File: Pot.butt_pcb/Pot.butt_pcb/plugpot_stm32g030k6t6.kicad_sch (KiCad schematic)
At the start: 12 parts, among them J1 Conn_01x04_Male, J2 Conn_01x05_Male, SW1 SW_Push, U1 STM32G030K6T6

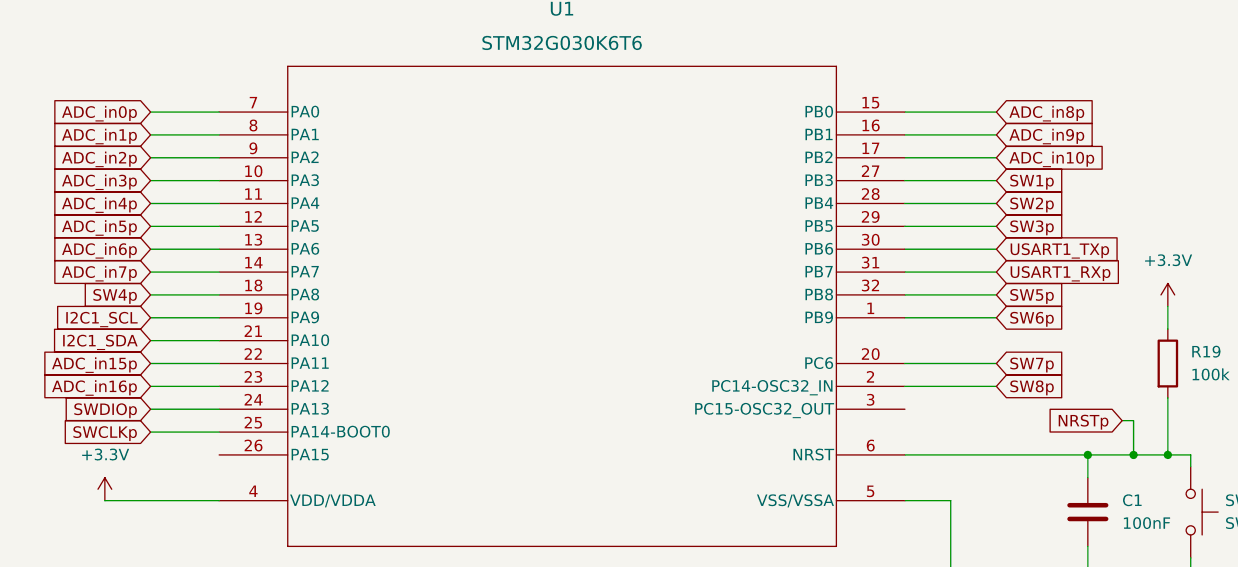
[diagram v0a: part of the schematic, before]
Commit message: Pot.but_pcb in progress
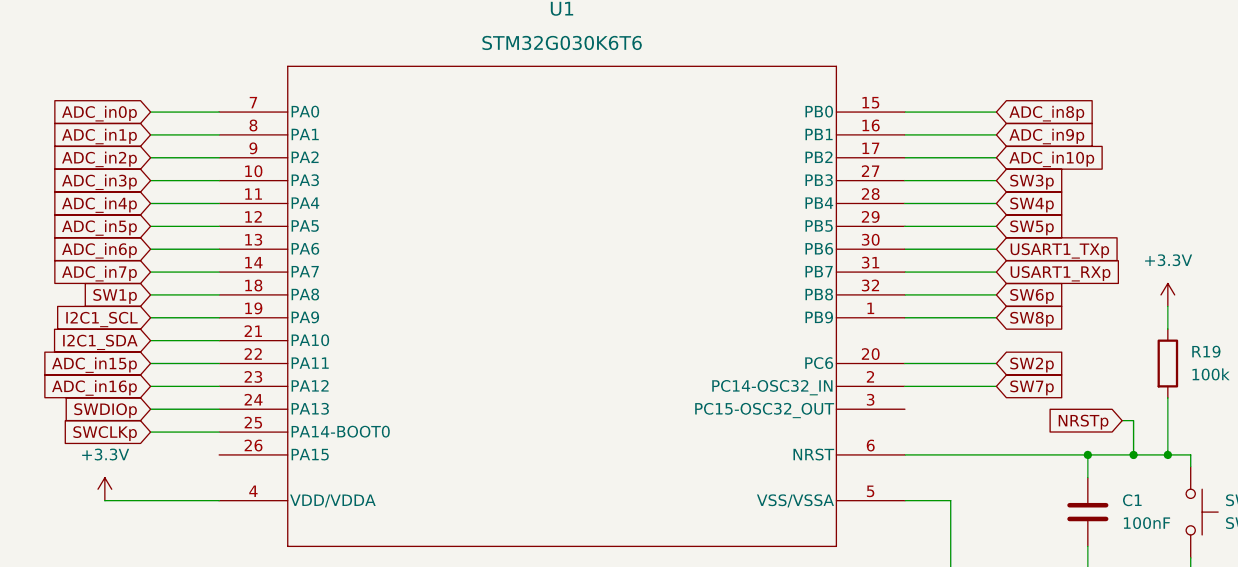
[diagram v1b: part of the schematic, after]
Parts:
- J1: footprint Connector_PinSocket_2.54mm:PinSocket_1x04_P2.54mm_Horizontal -> Connector_PinSocket_2.54mm:PinSocket_1x04_P2.54mm_Vertical
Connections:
- net SW1p: now also U1.18 (PA8); no longer U1.27 (PB3)
- net SW2p: now also U1.20 (PC6); no longer U1.28 (PB4)
- net SW3p: now also U1.27 (PB3); no longer U1.29 (PB5)
- net SW4p: now also U1.28 (PB4); no longer U1.18 (PA8)
- net SW5p: now also U1.29 (PB5); no longer U1.32 (PB8)
- net SW6p: now also U1.32 (PB8); no longer U1.1 (PB9)
- net SW7p: now also U1.2 (PC14-OSC32_IN); no longer U1.20 (PC6)
- net SW8p: now also U1.1 (PB9); no longer U1.2 (PC14-OSC32_IN)
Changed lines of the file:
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@@
     )
   )
-  (global_label "SW2p" (shape input) (at 137.16 60.96 0) (fields_autoplaced)
+  (global_label "SW4p" (shape input) (at 137.16 60.96 0) (fields_autoplaced)
     (effects (font (size 1.27 1.27)) (justify left))
     (property "Intersheet References" "${INTERSHEET_REFS}" (id 0) (at 144.5926 60.8806 0)
@@
     )
   )
-  (global_label "SW3p" (shape input) (at 137.16 63.5 0) (fields_autoplaced)
+  (global_label "SW5p" (shape input) (at 137.16 63.5 0) (fields_autoplaced)
     (effects (font (size 1.27 1.27)) (justify left))
     (property "Intersheet References" "${INTERSHEET_REFS}" (id 0) (at 144.5926 63.4206 0)
@@
     )
   )
-  (global_label "SW5p" (shape input) (at 137.16 71.12 0) (fields_autoplaced)
+  (global_label "SW6p" (shape input) (at 137.16 71.12 0) (fields_autoplaced)
     (effects (font (size 1.27 1.27)) (justify left))
     (property "Intersheet References" "${INTERSHEET_REFS}" (id 0) (at 144.5926 71.0406 0)
@@
     )
   )
-  (global_label "SW1p" (shape input) (at 137.16 58.42 0) (fields_autoplaced)
+  (global_label "SW3p" (shape input) (at 137.16 58.42 0) (fields_autoplaced)
     (effects (font (size 1.27 1.27)) (justify left))
     (property "Intersheet References" "${INTERSHEET_REFS}" (id 0) (at 144.5926 58.3406 0)
@@
     )
   )
-  (global_label "SW4p" (shape input) (at 43.18 71.12 180) (fields_autoplaced)
+  (global_label "SW1p" (shape input) (at 43.18 71.12 180) (fields_autoplaced)
     (effects (font (size 1.27 1.27)) (justify right))
     (property "Intersheet References" "${INTERSHEET_REFS}" (id 0) (at 35.7474 71.0406 0)
@@
     )
   )
-  (global_label "SW8p" (shape input) (at 137.16 81.28 0) (fields_autoplaced)
+  (global_label "SW7p" (shape input) (at 137.16 81.28 0) (fields_autoplaced)
     (effects (font (size 1.27 1.27)) (justify left))
     (property "Intersheet References" "${INTERSHEET_REFS}" (id 0) (at 144.5926 81.2006 0)
@@
     )
   )
-  (global_label "SW7p" (shape input) (at 137.16 78.74 0) (fields_autoplaced)
+  (global_label "SW2p" (shape input) (at 137.16 78.74 0) (fields_autoplaced)
     (effects (font (size 1.27 1.27)) (justify left))
     (property "Intersheet References" "${INTERSHEET_REFS}" (id 0) (at 144.5926 78.6606 0)
@@
     )
   )
-  (global_label "SW6p" (shape input) (at 137.16 73.66 0) (fields_autoplaced)
+  (global_label "SW8p" (shape input) (at 137.16 73.66 0) (fields_autoplaced)
     (effects (font (size 1.27 1.27)) (justify left))
     (property "Intersheet References" "${INTERSHEET_REFS}" (id 0) (at 144.5926 73.5806 0)
@@
     (property "Reference" "J1" (id 0) (at 219.075 88.9 0))
     (property "Value" "Conn_01x04_Male" (id 1) (at 219.075 91.44 0))
-    (property "Footprint" "Connector_PinSocket_2.54mm:PinSocket_1x04_P2.54mm_Horizontal" (id 2) (at 218.44 96.52 0)
-      (effects (font (size 1.27 1.27)) hide)
-    )
+    (property "Footprint" "Connector_PinSocket_2.54mm:PinSocket_1x04_P2.54mm_Vertical" (id 2) (at 218.44 96.52 0)
+      (effects (font (size 1.27 1.27)) hide)
+    )

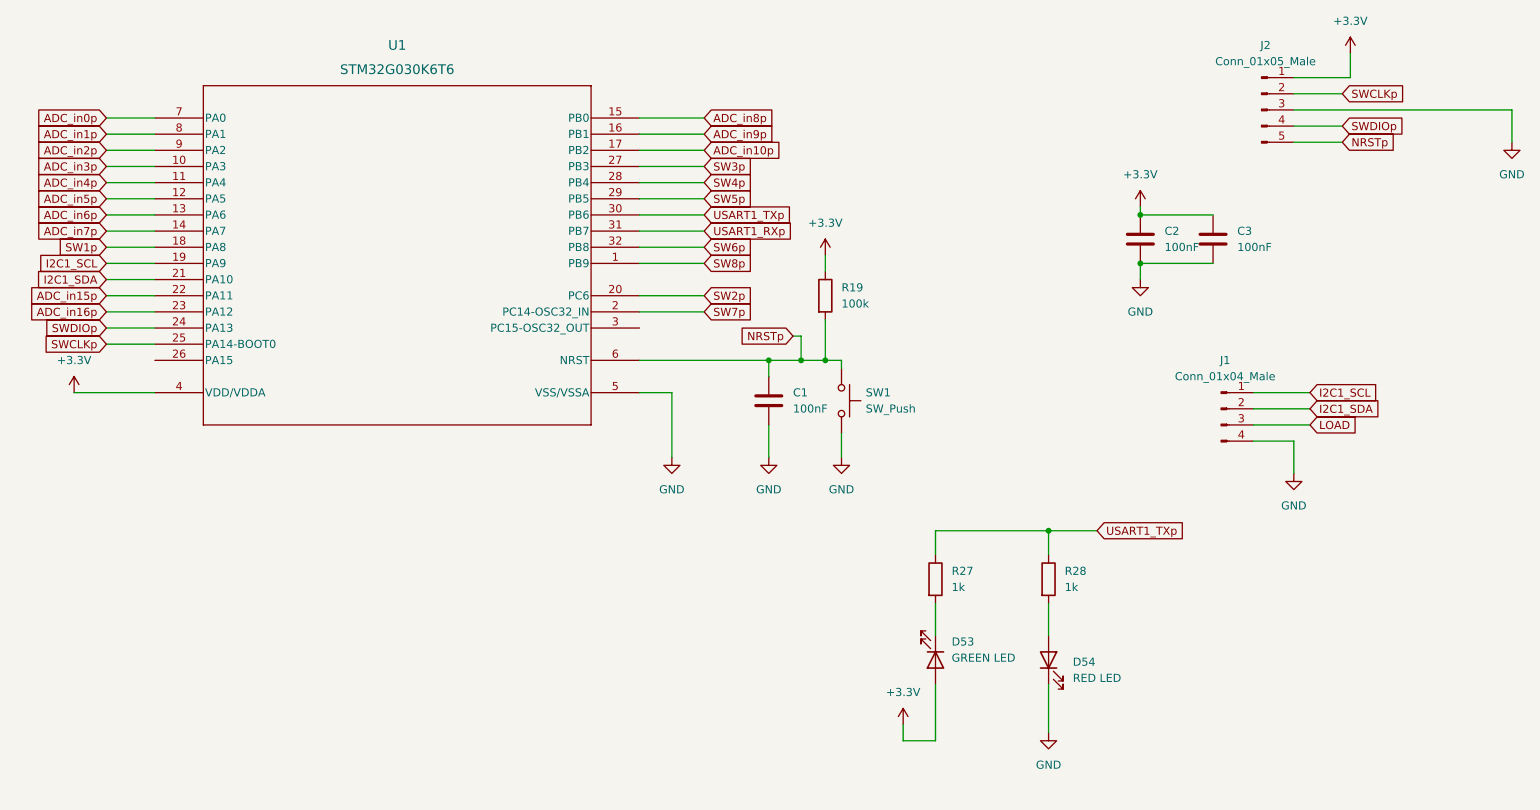
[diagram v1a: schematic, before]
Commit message: pcb design fixing
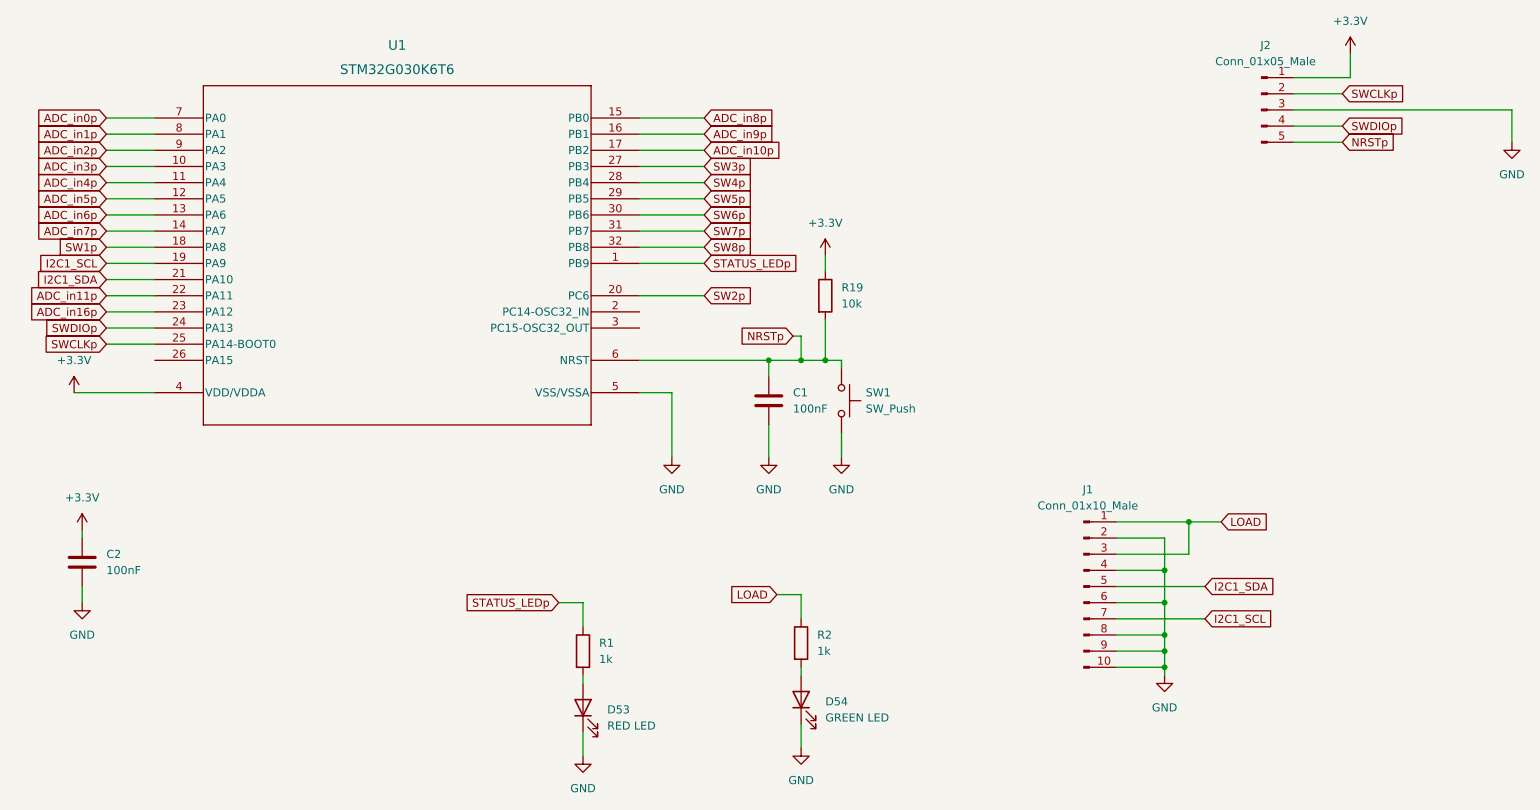
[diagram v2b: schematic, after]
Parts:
- removed C3: 100nF, Capacitor_SMD:C_0805_2012Metric_Pad1.18x1.45mm_HandSolder, symbol Device:C
- removed J1: Conn_01x04_Male, Connector_PinSocket_2.54mm:PinSocket_1x04_P2.54mm_Vertical, symbol Connector:Conn_01x04_Male
- removed R27, R28: 1k, Resistor_SMD:R_0805_2012Metric_Pad1.20x1.40mm_HandSolder, symbol Device:R
- added J1: Conn_01x10_Male, Connector_IDC:IDC-Header_2x05_P2.54mm_Horizontal, symbol Connector:Conn_01x10_Male
- added R1, R2: 1k, Resistor_SMD:R_0805_2012Metric_Pad1.20x1.40mm_HandSolder, symbol Device:R
- D53: value GREEN LED -> RED LED
- D54: value RED LED -> GREEN LED
- R19: value 100k -> 10k
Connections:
- net USART1_RXp is gone; now on net SW7p: U1.31 (PB7)
- net USART1_TXp is gone; now on net SW6p: U1.30 (PB6)
- net +3V3: no longer D53.2 (A)
- net GND: now also D53.1 (K), J1.10 (Pin_10), J1.2 (Pin_2), J1.4 (Pin_4), J1.6 (Pin_6), J1.8 (Pin_8), J1.9 (Pin_9)
- net I2C1_SCL: now also J1.7 (Pin_7)
- net I2C1_SDA: now also J1.5 (Pin_5)
- net LOAD: now also J1.1 (Pin_1), J1.3 (Pin_3), R2.1
- net SW6p: no longer U1.32 (PB8)
- net SW7p: no longer U1.2 (PC14-OSC32_IN)
- net SW8p: now also U1.32 (PB8); no longer U1.1 (PB9)
- net at D54.2 (A): now also R2.2
- net ADC_in15p renamed ADC_in11p
- new net: D53.2 (A), R1.2
- new net STATUS_LEDp: R1.1, U1.1 (PB9)
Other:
- moved on the sheet: C2
